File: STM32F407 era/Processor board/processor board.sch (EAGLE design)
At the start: 41 parts, among them IC1 REG1117, U2 MAX13052ESA+, X1 MINI-USB-SCHIELD-32005-201, X2 057-010-1, Y1 25 MHz, Y2 32.768KHz

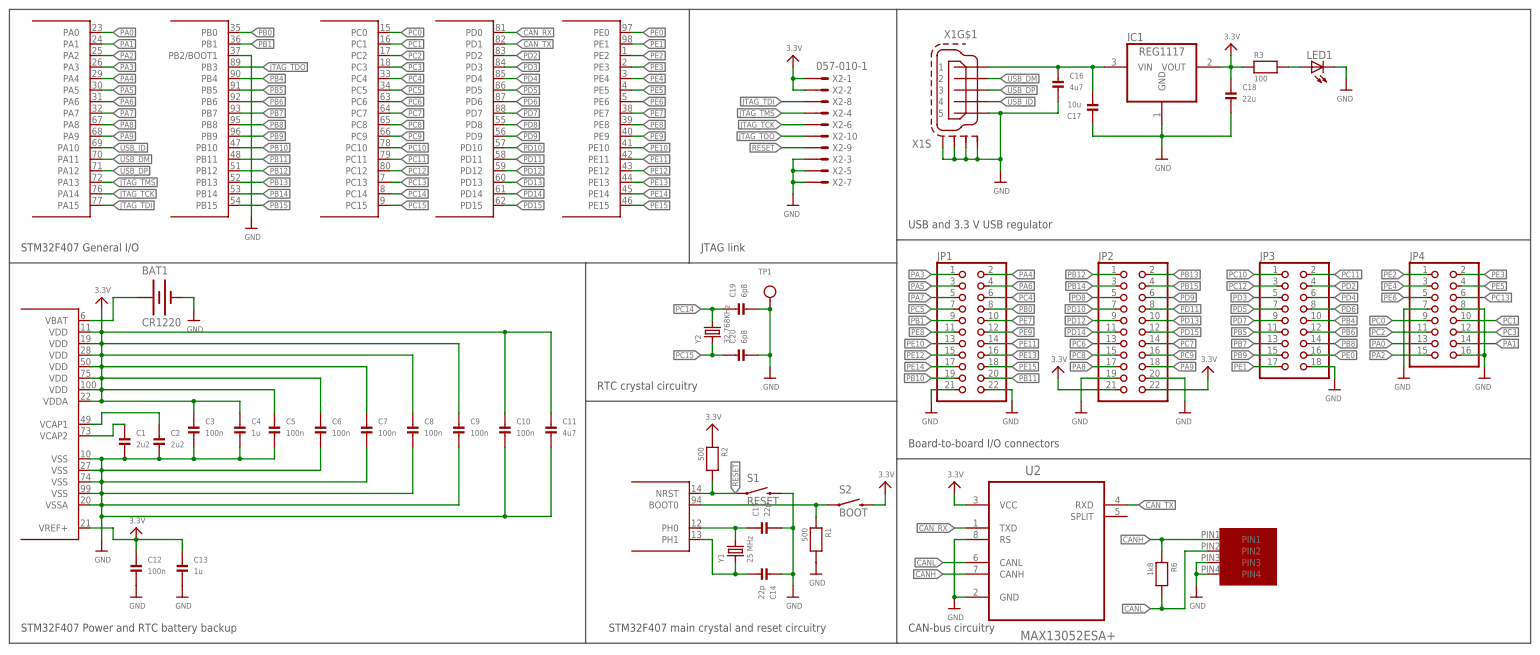
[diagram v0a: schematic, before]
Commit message: last layout update for V1
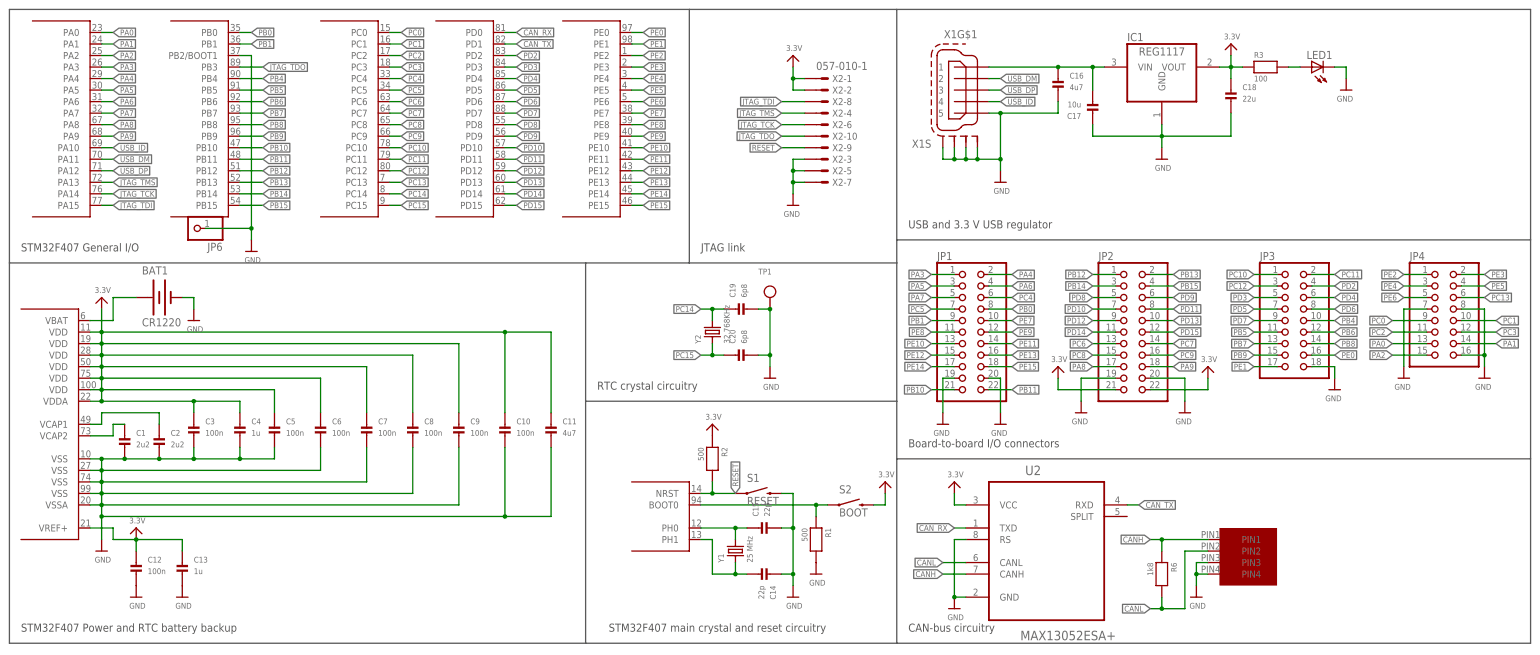
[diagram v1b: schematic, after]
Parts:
- added JP6: (no value), pinhead:PINHD-1X1
- C1, C10, C11, C12, C13, C14, C15, C19, C2, C20, C3, C4, C5, C6, C7, C8, C9: device microbuilder:CAP_CERAMIC_0402MP -> microbuilder:CAP_CERAMIC_0603MP
- R1, R2, R3, R6: device microbuilder:RESISTOR_0402MP -> microbuilder:RESISTOR_0603MP
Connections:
- net GND: now also JP1.19, JP1.20, JP6.1; no longer JP1.21, JP1.22
- net PB10: now also JP1.21; no longer JP1.19
- net PB11: now also JP1.22; no longer JP1.20
